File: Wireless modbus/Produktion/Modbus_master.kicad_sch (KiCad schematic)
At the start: 75 parts, among them IC1 LoRa-E5, J1 Screw_Terminal_01x03, J2 SIM8066-6-1-14-01-A, J3 Conn_01x04_Pin, J4 Conn_Coaxial, J5 Screw_Terminal_01x04, J6 AVR-ISP-6, Q1 BC847CW, Q2 BC847CW, SW1 TL3305AF260QG, U1 ATmega2560-16A, U2 SP485EN-L/TR, U3 L7805, U4 SIM7080G, U5 LSF0204PW-Q100J, Y1 ABM3B-8.000MHZ-10-1-U-T

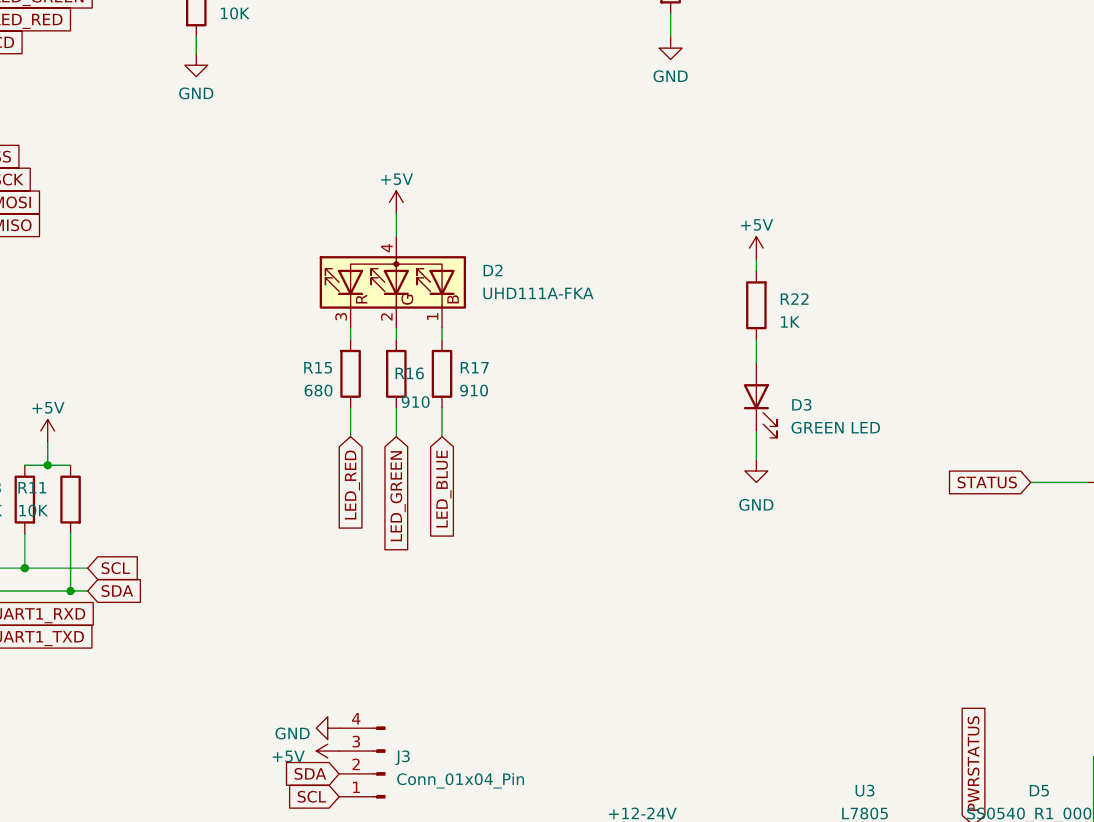
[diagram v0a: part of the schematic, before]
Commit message: Ændring
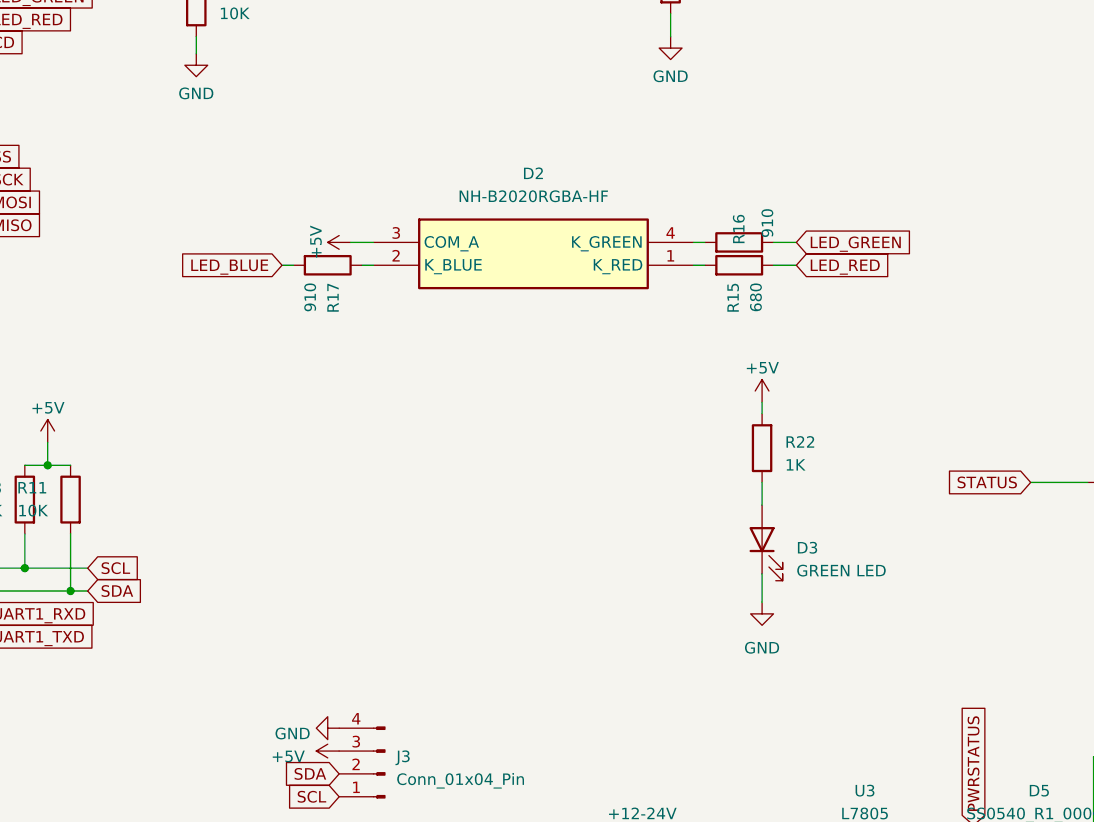
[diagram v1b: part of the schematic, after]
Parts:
- removed D2: UHD111A-FKA, LED_SMD_RGB:LED_RGB_1_1_mm, symbol Device:LED_BGRA
- added D2: NH-B2020RGBA-HF, NHB2020RGBAHF, symbol SamacSys_Parts:NH-B2020RGBA-HF
- J2: JLCPART# (none) -> C381071
- J4: JLCPART# (none) -> C434808
- Q1, Q2: JLCPART# (none) -> C75567
- R1, R11, R12, R13, R14, R18, R19, R21, R26, R27, R29, R30, R5, R6, R7, R8, R9: JLCPART# (none) -> C25744
- R10: JLCPART# (none) -> C25792
- R15: JLCPART# (none) -> C25113
- R16, R17: JLCPART# (none) -> C44933
- R2, R3, R4: JLCPART# (none) -> C25092
- R20: JLCPART# (none) -> C25765
- R22, R23, R25: JLCPART# (none) -> C11702
- R24: JLCPART# (none) -> C560547
- R28: JLCPART# (none) -> C25764
- SW1: JLCPART# (none) -> C2886902
- U1: JLCPART# (none) -> C22460
- U2: JLCPART# (none) -> C6855
- U4: JLCPART# (none) -> C2943992
- U5: JLCPART# (none) -> C202288
- Y1: JLCPART# (none) -> C276420
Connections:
- net VCC_5: now also D2.3 (COM_A)
- net at R17.1: now also D2.2 (K_BLUE)
- net at R16.2: now also D2.4 (K_GREEN)
- net at R15.2: now also D2.1 (K_RED)
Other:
- moved on the sheet: D3, R15, R16, R17, R22
